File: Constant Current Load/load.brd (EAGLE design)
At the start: 145 x 63.5 mm, 51 parts

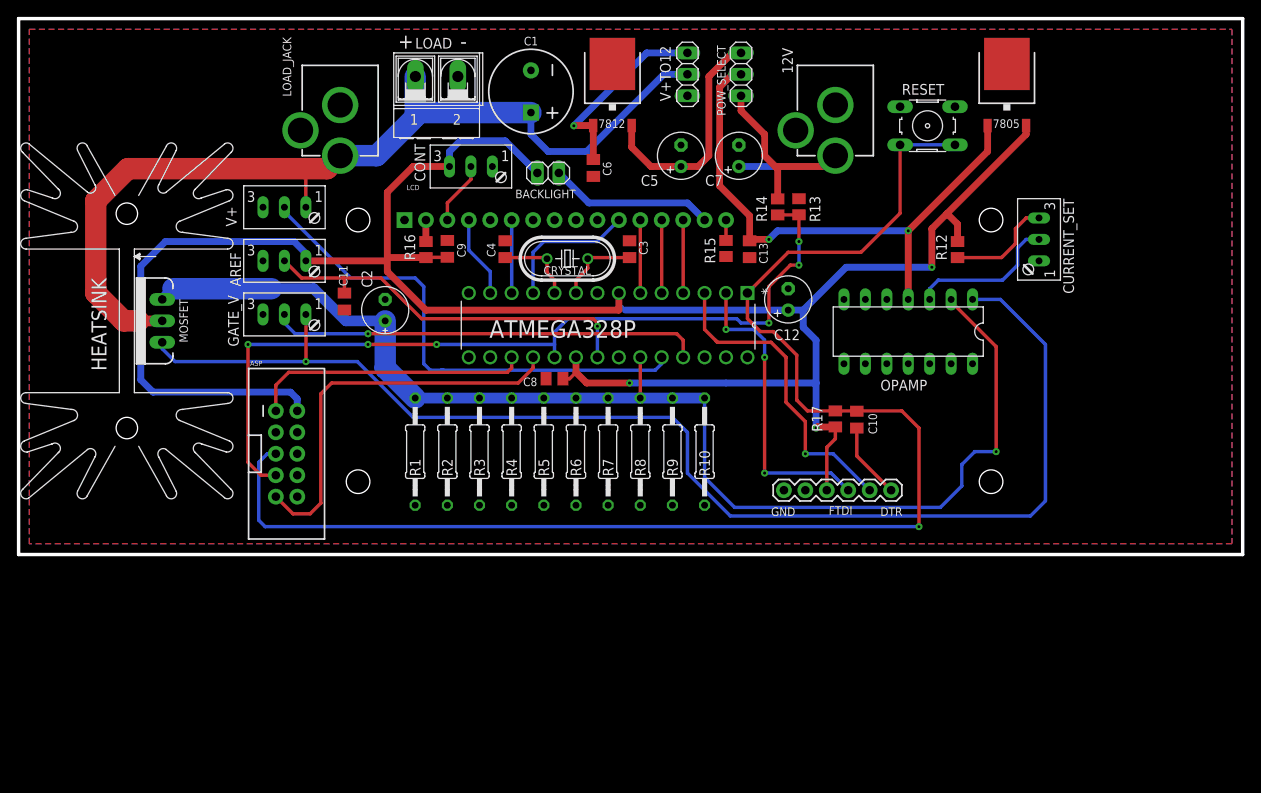
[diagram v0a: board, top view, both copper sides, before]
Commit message: Final
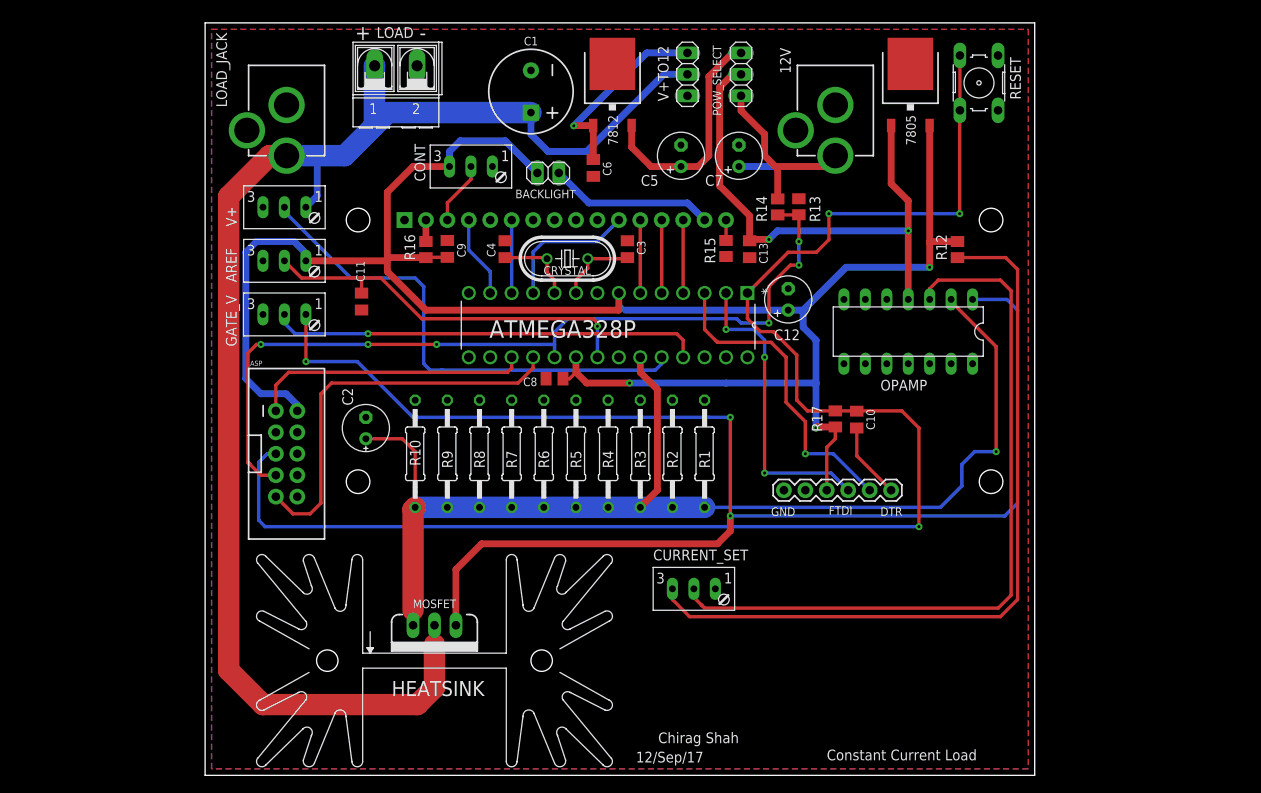
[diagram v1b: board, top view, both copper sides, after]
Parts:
- moved CURRENT_SET 58.2 mm to (64.5, 4.83), turned to 0 degrees
- moved HEATSINK 53.1 mm to (33.8, -1.52), turned to 0 degrees
- moved MOSFET 48.4 mm to (33.8, 1.78), turned to 180 degrees
- moved R5 34.3 mm to (65.8, 22.1), turned to 270 degrees
- moved R7 34.3 mm to (31.5, 22.1), turned to 270 degrees
- moved R10 26.7 mm to (62.0, 22.1), turned to 270 degrees
- moved R9 26.7 mm to (35.3, 22.1), turned to 270 degrees
- moved R3 19.1 mm to (39.1, 22.1), turned to 270 degrees
- moved R8 19.1 mm to (58.2, 22.1), turned to 270 degrees
- moved C2 14.2 mm to (25.7, 25.1)
- moved R1 11.4 mm to (42.9, 22.1), turned to 270 degrees
- moved R6 11.4 mm to (54.4, 22.1), turned to 270 degrees
- moved 7805 11.4 mm to (90.2, 65.8)
- moved RESET 7.94 mm to (98.3, 66.0), turned to 270 degrees
- moved LOAD_JACK 6.35 mm to (16.3, 71.1)
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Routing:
- net N$9: track 12.6 -> 90.7 mm
- net N$1: track 17.8 -> 87.9 mm
- net V+: track 111.8 -> 169.9 mm
- net +5V: track 260.7 -> 230.9 mm
- net GATE_V: track 152.2 -> 176.5 mm, vias 1 -> 3
- net RESET: track 168.1 -> 181.0 mm, vias 1 -> 3
- net V_ACC_RESISTOR: track 148.1 -> 139.9 mm
- net +12V: track 66.6 -> 63.5 mm
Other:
- board size 145 x 63.5 mm -> 98.3 x 89.2 mm
- board text added: "12/Sep/17"
- board text added: "Chirag Shah"
- board text added: "Constant Current Load"
